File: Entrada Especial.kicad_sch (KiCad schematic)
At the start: 57 parts, among them U28 TLV9301xDBV, U29 TLV9301xDBV, U30 LM7705, U31 MCP1799T-5002H/TT

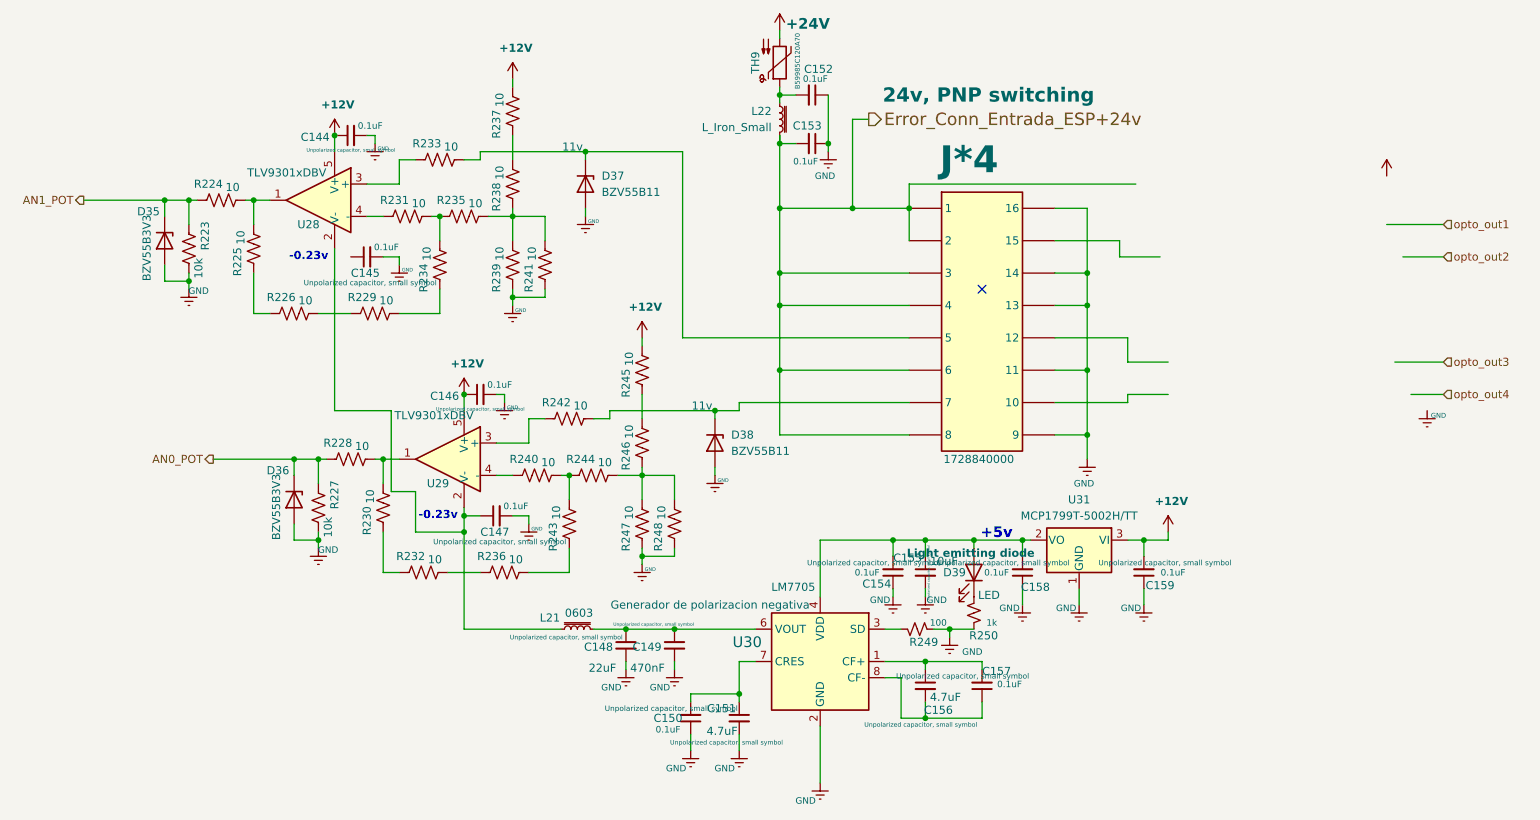
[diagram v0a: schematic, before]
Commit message: 05/06/26
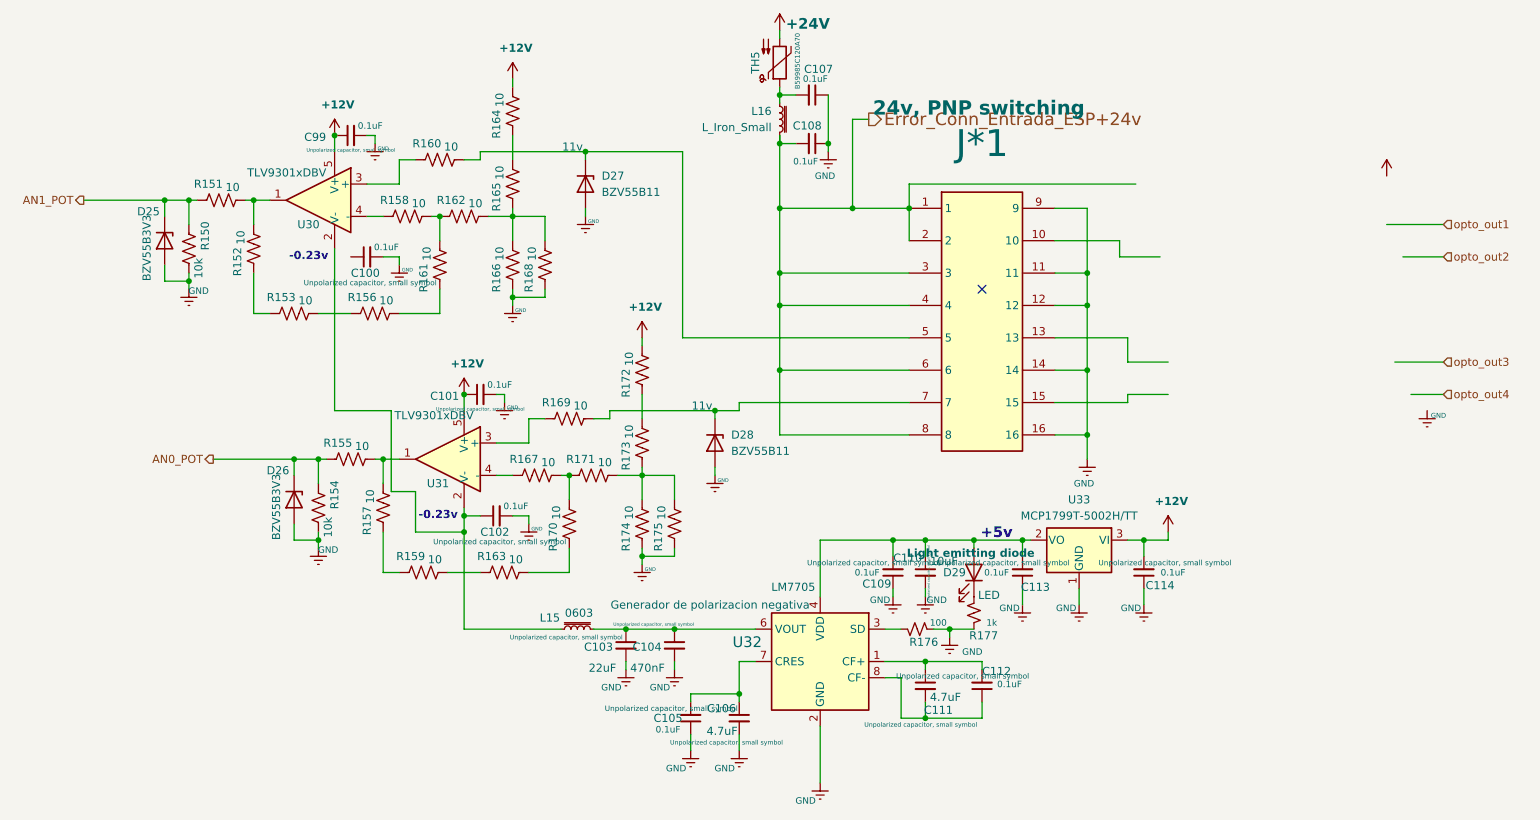
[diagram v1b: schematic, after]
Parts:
- removed J*4: 1728840000, CONECTORES GRACIDA:16POS-2LINEAS-3.5PITCH, symbol CONECTORES GRACIDA:Weidmüller 1728840000 16pos P3.5mm socket
- added J*1: 1728840000, CONECTORES GRACIDA:16POS-2LINEAS-3.5PITCH, symbol CONECTORES GRACIDA:1728840000_1
- renumbered C145 to C100, C146 to C101, C147 to C102, C148 to C103, C149 to C104, C150 to C105, C151 to C106, C152 to C107, C153 to C108, C154 to C109, C155 to C110, C156 to C111, C157 to C112, C158 to C113, C159 to C114, C144 to C99, D35 to D25, D36 to D26, D37 to D27, D38 to D28, D39 to D29, L21 to L15, L22 to L16, R223 to R150, R224 to R151, R225 to R152, R226 to R153, R227 to R154, R228 to R155, R229 to R156, R230 to R157, R231 to R158, R232 to R159, R233 to R160, R234 to R161, R235 to R162, R236 to R163, R237 to R164, R238 to R165, R239 to R166, R240 to R167, R241 to R168, R242 to R169, R243 to R170, R244 to R171, R245 to R172, R246 to R173, R247 to R174, R248 to R175, R249 to R176, R250 to R177, TH9 to TH5, U28 to U30, U29 to U31, U30 to U32, U31 to U33
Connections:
- net Error_Conn_Entrada_ESP+24v: now also J*1.1, J*1.2, J*1.3, J*1.4, J*1.6, J*1.8
- net GND: now also J*1.11, J*1.12, J*1.14, J*1.16, J*1.9
- net at D27.1 (K), R160.1: now also J*1.5
- net at D28.1 (K), R169.1: now also J*1.7

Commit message: 08-06-26
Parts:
- U30, U31: footprint Package_TO_SOT_SMD:SOT-23-5 -> Package_TO_SOT_SMD:SOT-23-5_HandSoldering
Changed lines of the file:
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@@
 			)
 		)
-		(property "Footprint" "Package_TO_SOT_SMD:SOT-23-5"
+		(property "Footprint" "Package_TO_SOT_SMD:SOT-23-5_HandSoldering"
 			(at 97.79 123.19 0)
 			(effects
@@
 			)
 		)
-		(property "Footprint" "Package_TO_SOT_SMD:SOT-23-5"
+		(property "Footprint" "Package_TO_SOT_SMD:SOT-23-5_HandSoldering"
 			(at 77.47 82.55 0)
 			(effects
